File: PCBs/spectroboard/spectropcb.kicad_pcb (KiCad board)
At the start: 2 copper layers, 67.5 x 50 mm, 14 parts, among them J1 Conn_02x07_Odd_Even, J2 Conn_02x08_Odd_Even, J3 Conn_02x08_Odd_Even, J4 Conn_01x02_Pin, J6 SM04B-GHS-TB, Q1 2SA1015, U1 TCD1304DG, U2 SN74HC04N

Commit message: first thoughts
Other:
- board text added: "How big are these devices, the motherboard has an overhang past the jumpers, so if these are tall it could be an issue"
- board text added: "I would reccomend using a ground plane and vias instead of the ground traces, especially since most of the traces on the back are ground anyways"
- board text added: "Pretty jaggad traces, not a huge deal but there is space, so I'd change it"
- board text added: "This jumper is backwards"
- board text added: "this traces doesn't need to go around, it can just go straight to its destination, since its on the bottom"
- board text added: "use JST GH, not PH"
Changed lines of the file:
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@@
 		(layer "Edge.Cuts")
+	)
+	(gr_rect
+		(start 119.08 50.01)
+		(end 132.43 63.45)
+		(stroke
+			(width 0.1)
+			(type default)
+		)
+		(fill no)
+		(layer "User.1")
+	)
+	(gr_text "I would reccomend using a ground plane \nand vias instead of the ground traces, especially since most of the\ntraces on the back are ground anyways"
+		(at 146.08 41.93 0)
+		(layer "User.1")
+		(effects
+			(font
+				(size 1 1)
+				(thickness 0.15)
+			)
+			(justify left bottom)
+		)
+	)
+	(gr_text "This jumper is backwards"
+		(at 127.4 93.98 0)
+		(layer "User.1")
+		(effects
+			(font
+				(size 0.5 0.5)
+				(thickness 0.125)
+				(bold yes)
+			)
+			(justify left bottom)
+		)
+	)
+	(gr_text "use JST GH, not PH"
+		(at 146.99 89.89 0)
+		(layer "User.1")
+		(effects
+			(font
+				(size 0.5 0.5)
+				(thickness 0.125)
+				(bold yes)
+			)
+			(justify left bottom)
+		)
+	)
+	(gr_text "this traces doesn't need to go around, \nit can just go straight to its \ndestination, since its on the bottom\n"
+		(at 122.06 66.63 270)
+		(layer "User.1")
+		(effects
+			(font
+				(size 0.5 0.5)
+				(thickness 0.125)
+				(bold yes)
+			)
+			(justify left bottom)
+		)
+	)
+	(gr_text "Pretty jaggad traces,\nnot a huge deal but there\nis space, so I'd change it"
+		(at 119.08 54.54 0)
+		(layer "User.1")
+		(effects
+			(font
+				(size 1 1)
+				(thickness 0.15)
+			)
+			(justify left bottom)
+		)
+	)
+	(gr_text "How big are these devices, the \nmotherboard has an overhang past\nthe jumpers, so if these are tall\nit could be an issue"
+		(at 160.67 56.37 0)
+		(layer "User.1")
+		(effects
+			(font
+				(size 1 1)
+				(thickness 0.15)
+			)
+			(justify left bottom)
+		)
 	)
 	(segment

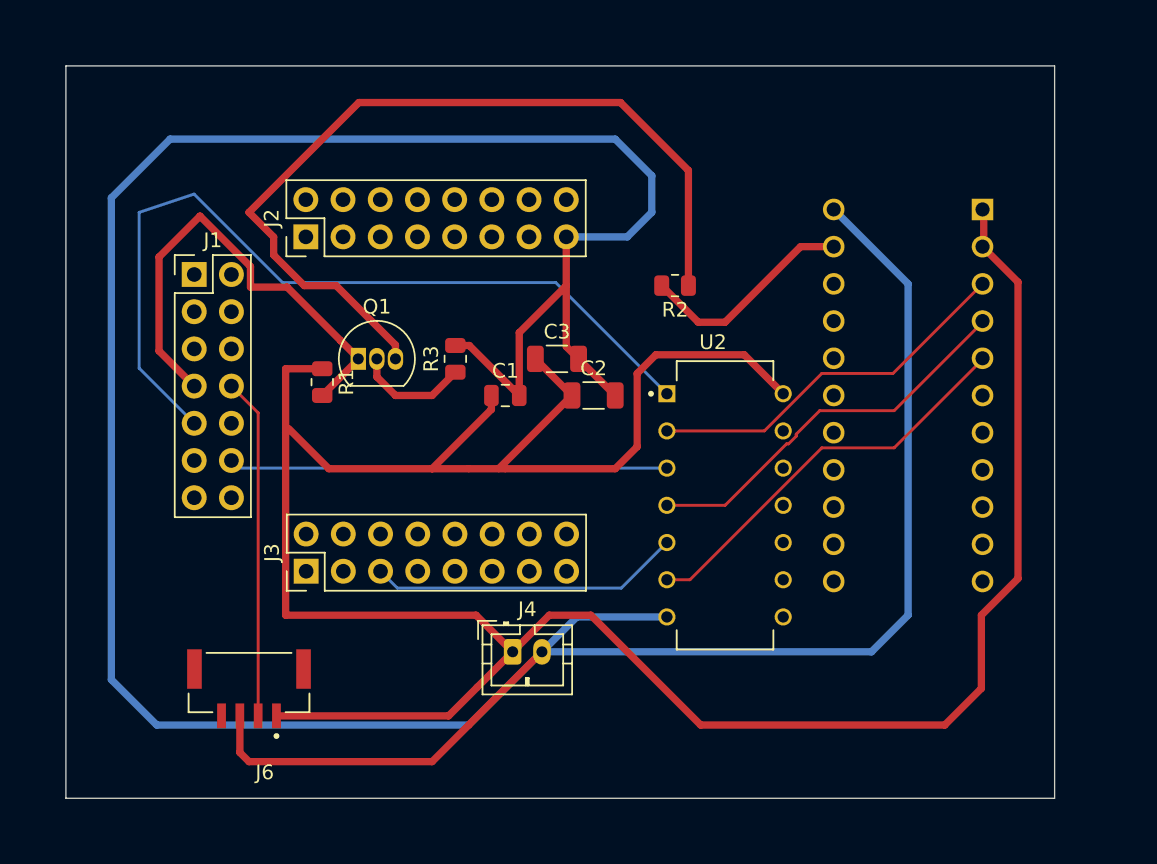
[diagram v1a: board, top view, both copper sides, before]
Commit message: updated pcb
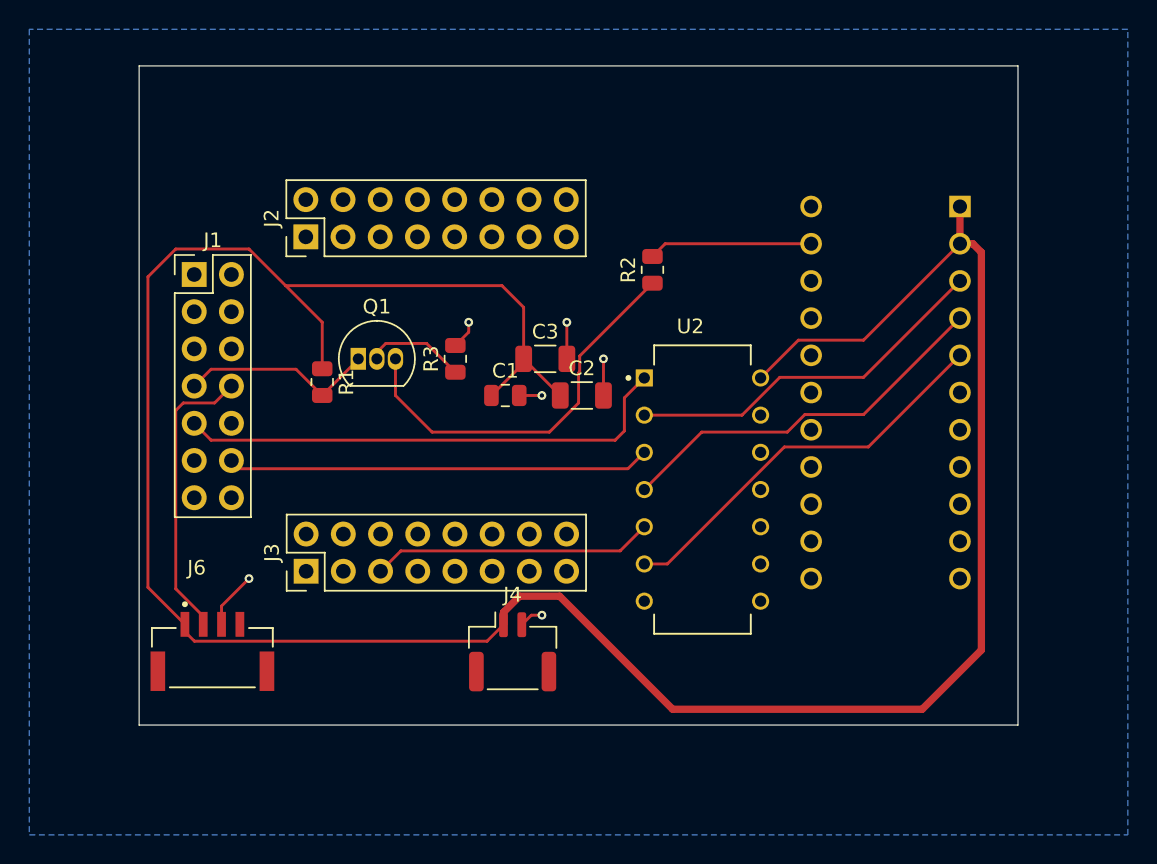
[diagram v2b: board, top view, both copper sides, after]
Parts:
- J4: footprint Connector_JST:JST_PH_B2B-PH-K_1x02_P2.00mm_Vertical -> Connector_JST:JST_GH_SM02B-GHS-TB_1x02-1MP_P1.25mm_Horizontal
- moved J6 3.54 mm to (127.5, 85.0), turned to 0 degrees
- moved R2 1.88 mm to (157.5, 58.9), turned to 90 degrees
- moved U2 1.88 mm to (161.0, 73.9)
- moved U1 1.56 mm to (178.5, 54.6)
- moved C2 0.80 mm to (152.7, 67.5)
- moved C3 0.80 mm to (150.2, 65.0)
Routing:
- net GND: track 232.9 -> 14.1 mm, vias 0 -> 6
- net Net-(Q1-B): track 58.3 -> 27.1 mm
- net /21: track 57.8 -> 34.3 mm
- net /17: track 33.0 -> 13.5 mm
- net +5V: track 185.8 -> 180.6 mm
- net Net-(U1-OS): track 14.9 -> 11.2 mm
- net /16: track 23.3 -> 19.9 mm
- net /39: track 21.3 -> 19.3 mm
- net Net-(Q1-C): track 8.00 -> 7.09 mm
- net Net-(U1-phiM): track 26.9 -> 26.4 mm
- added copper zone on B.Cu, net GND
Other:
- board size 67.5 x 50 mm -> 60 x 45 mm
- board text removed: "How big are these devices, the motherboard has an overhang past the jumpers, so if these are tall it could be an issue"
- board text removed: "I would reccomend using a ground plane and vias instead of the ground traces, especially since most of the traces on the back are ground anyways"
- board text removed: "Pretty jaggad traces, not a huge deal but there is space, so I'd change it"
- board text removed: "This jumper is backwards"
- board text removed: "this traces doesn't need to go around, it can just go straight to its destination, since its on the bottom"
- board text removed: "use JST GH, not PH"
